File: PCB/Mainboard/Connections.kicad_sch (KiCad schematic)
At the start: 37 parts, among them J10 I2C, J11 Servo 0, J12 Servo 1, J13 PW_IO_bak, J14 PW_IO_bak, J15 Servo 4, J16 Servo 5, J17 Servo 2, J18 Servo 3, J19 Servo 6, J2 BME680, J20 Servo 7, J3 GPIO, J4 PW_5V, J5 PW_3V3, J6 Micro_SD_Card_Det_Hirose_DM3AT, J7 Stepper_1, J8 Stepper_2, J9 SPI

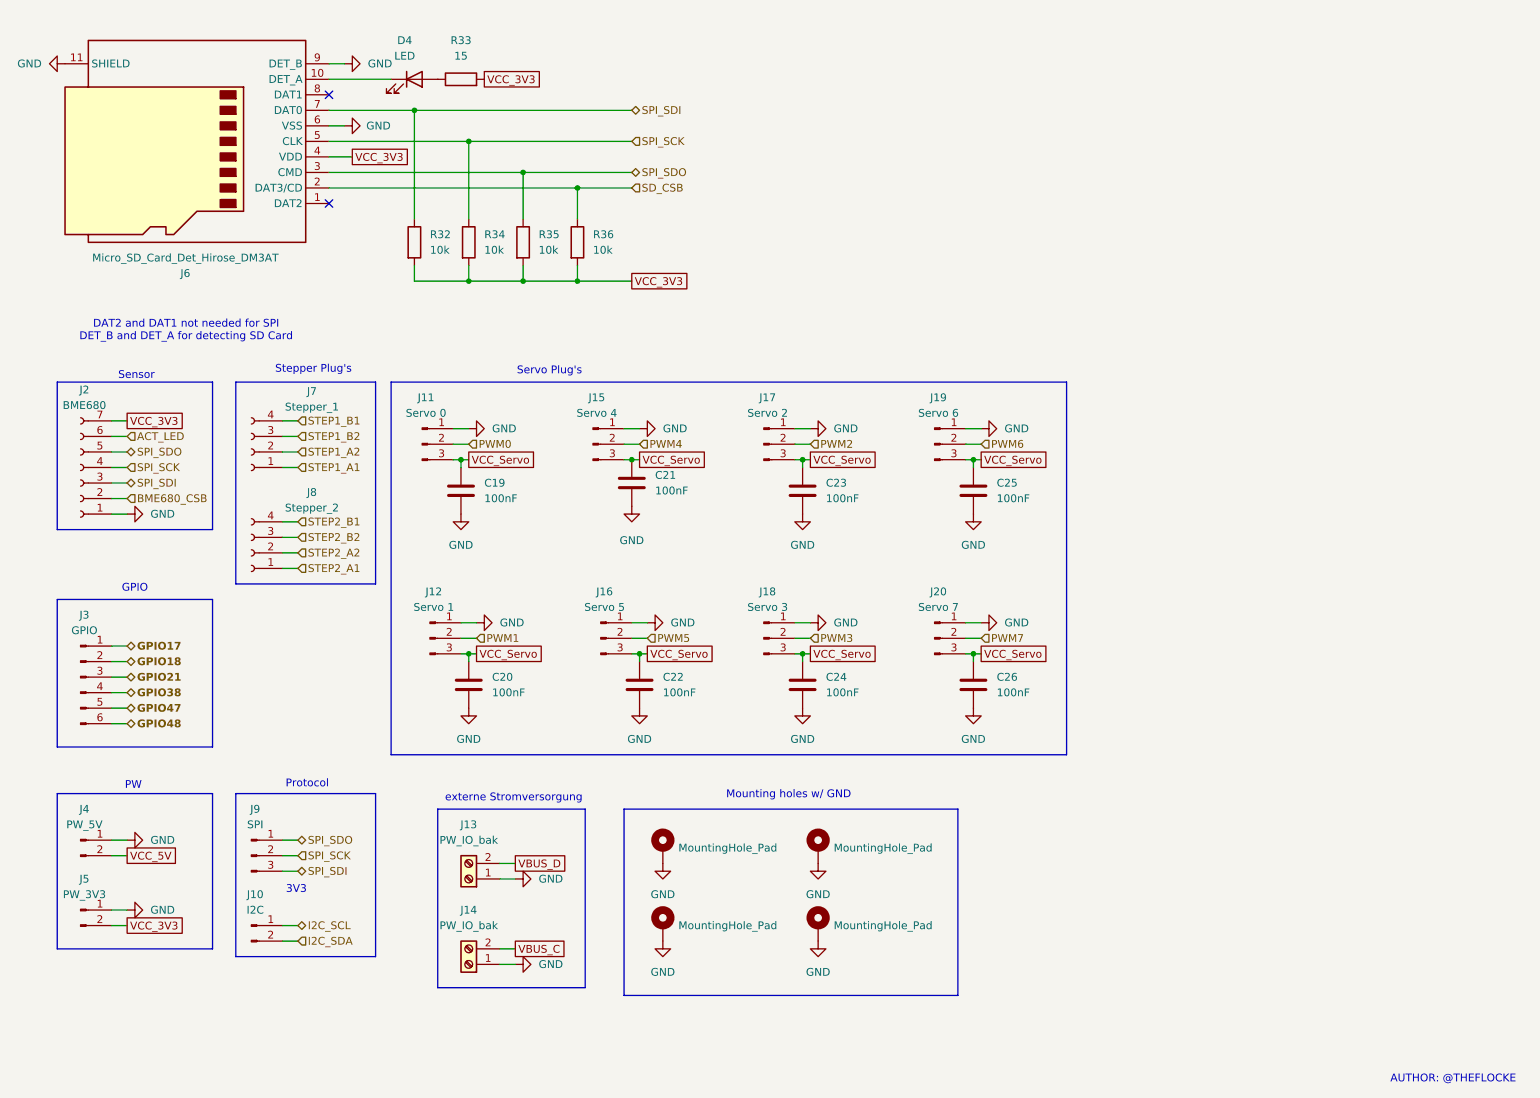
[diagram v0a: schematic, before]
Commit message: Fixed Grammar
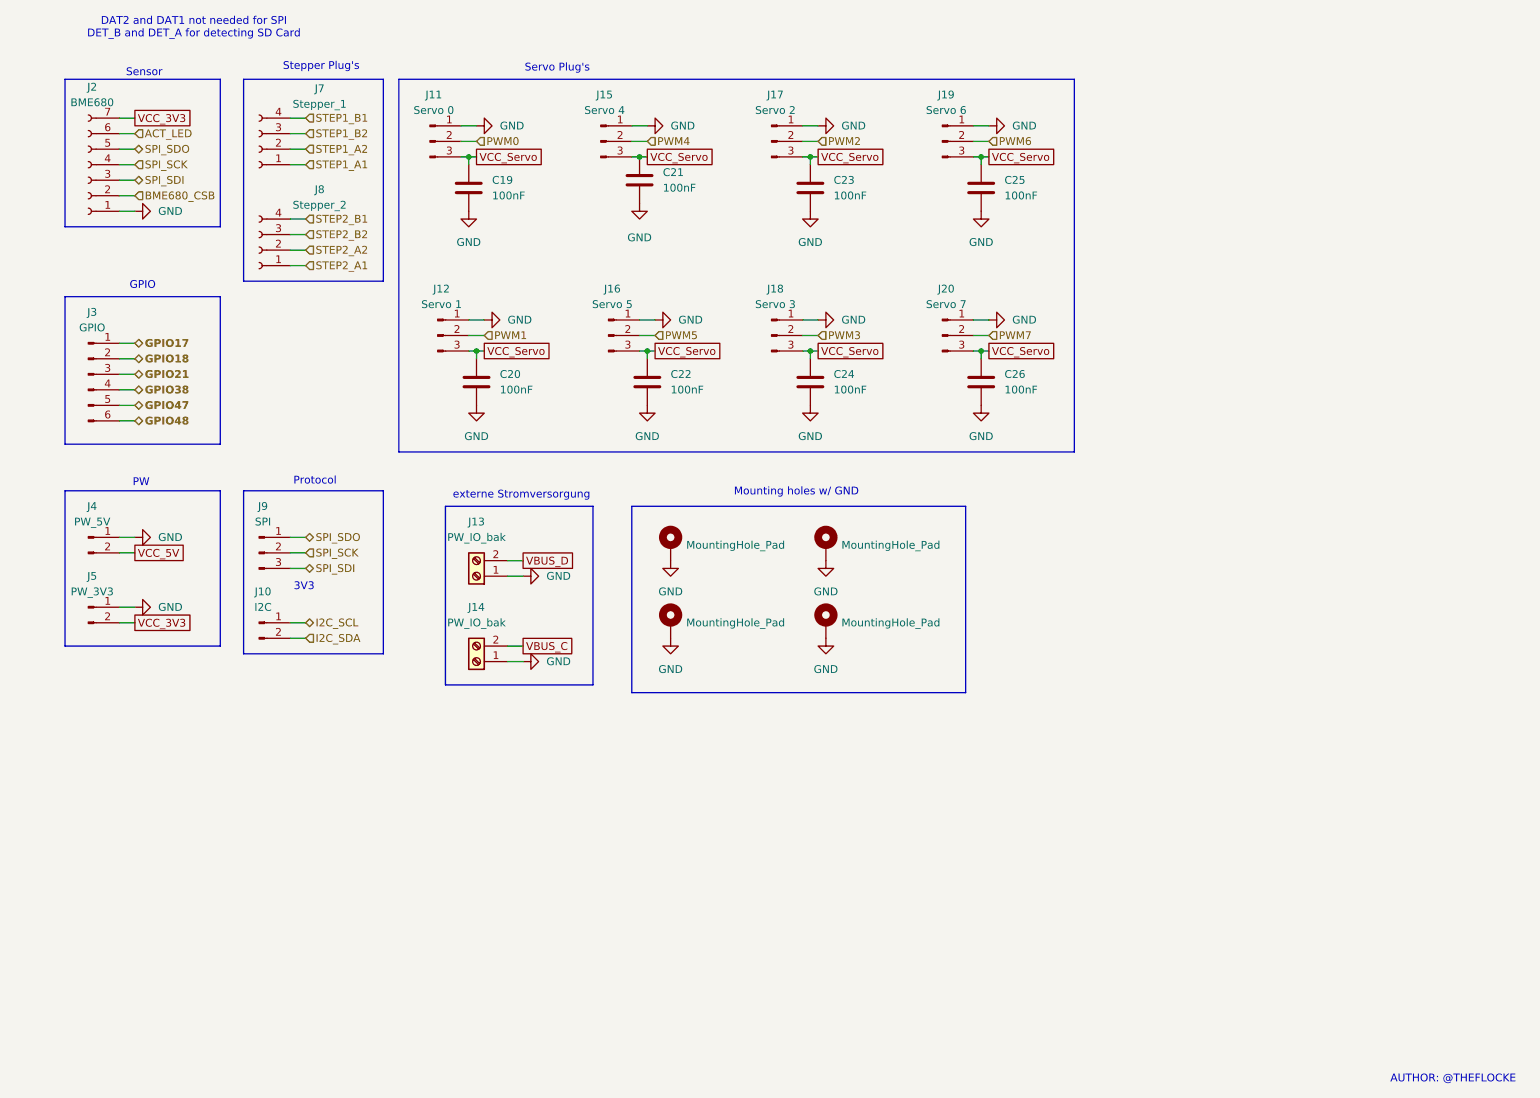
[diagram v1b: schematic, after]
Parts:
- removed D4: LED, Diode_SMD:D_0805_2012Metric_Pad1.15x1.40mm_HandSolder, symbol Device:LED
- removed J6: Micro_SD_Card_Det_Hirose_DM3AT, Connector_Card:microSD_HC_Hirose_DM3D-SF, symbol Connector:Micro_SD_Card_Det_Hirose_DM3AT
- removed R32, R34, R35, R36: 10k, Resistor_SMD:R_0805_2012Metric_Pad1.20x1.40mm_HandSolder, symbol Device:R
- removed R33: 15, Resistor_SMD:R_0805_2012Metric_Pad1.20x1.40mm_HandSolder, symbol Device:R
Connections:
- no-connect marks 2 -> 0
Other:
- moved on the sheet: C19, C20, C21, C22, C23, C24, C25, C26, J10, J11, J12, J13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

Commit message: upload images and deleted pcb new
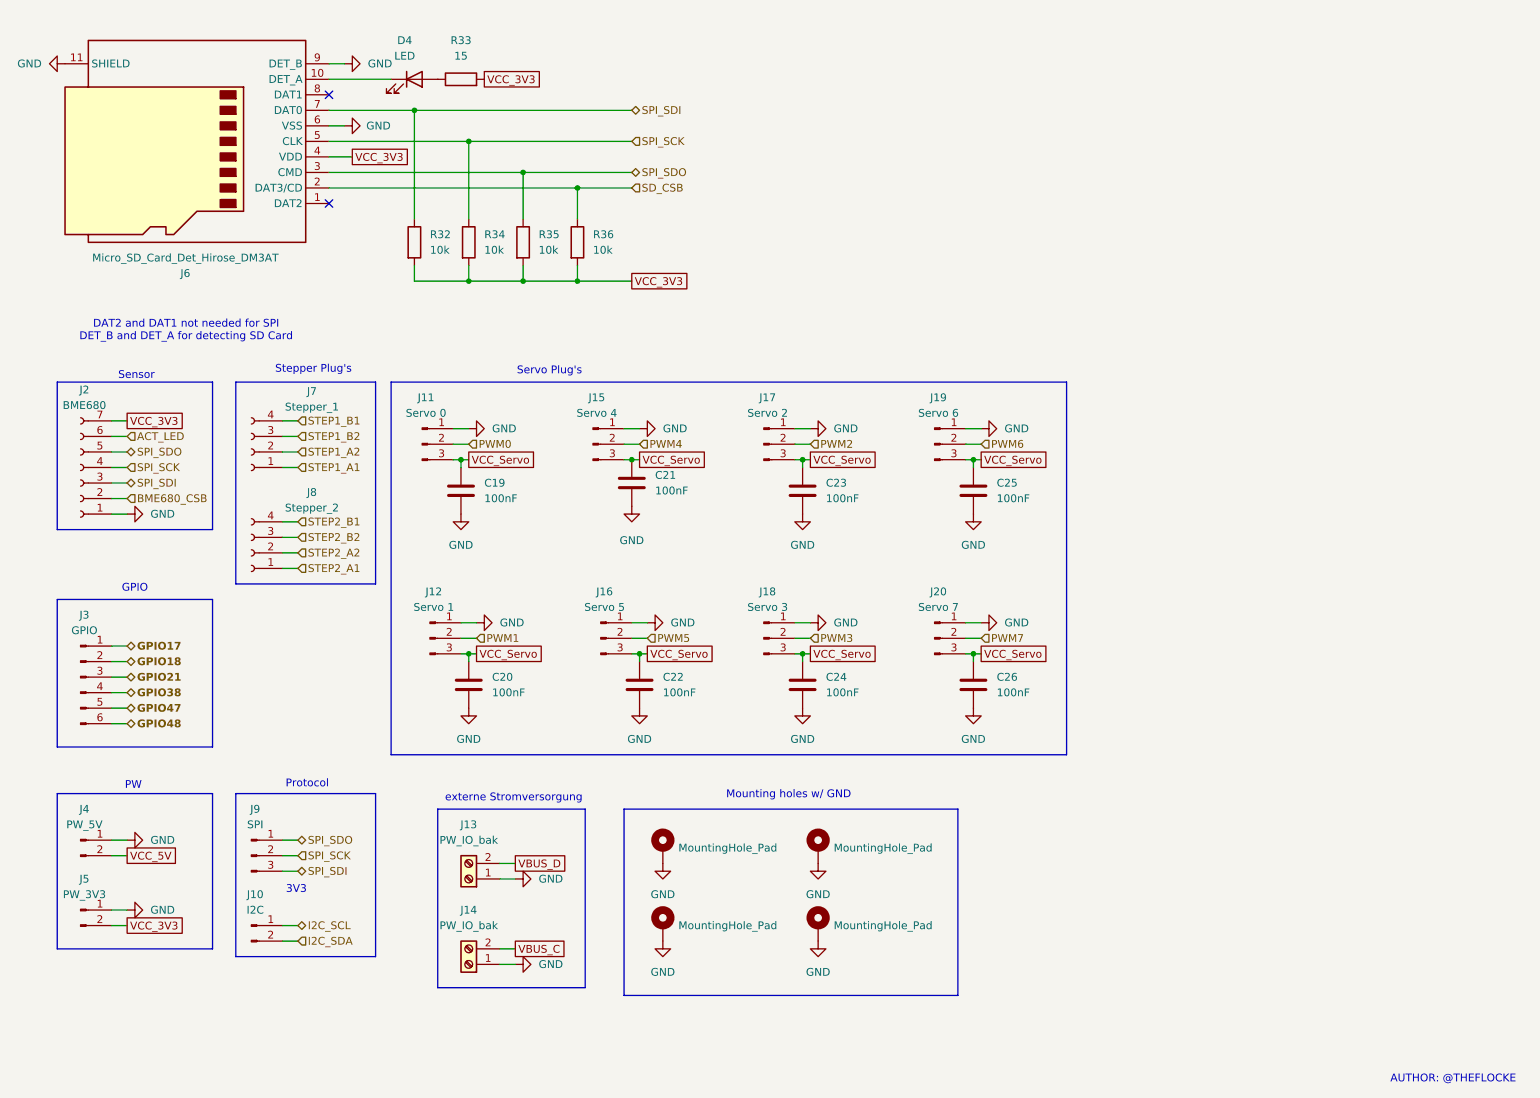
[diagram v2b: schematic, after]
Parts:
- added D4: LED, Diode_SMD:D_0805_2012Metric_Pad1.15x1.40mm_HandSolder, symbol Device:LED
- added J6: Micro_SD_Card_Det_Hirose_DM3AT, Connector_Card:microSD_HC_Hirose_DM3D-SF, symbol Connector:Micro_SD_Card_Det_Hirose_DM3AT
- added R32, R34, R35, R36: 10k, Resistor_SMD:R_0805_2012Metric_Pad1.20x1.40mm_HandSolder, symbol Device:R
- added R33: 15, Resistor_SMD:R_0805_2012Metric_Pad1.20x1.40mm_HandSolder, symbol Device:R
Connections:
- net GND: now also J6.11 (SHIELD), J6.6 (VSS), J6.9 (DET_B)
- net SPI_SCK: now also J6.5 (CLK), R34.1
- net SPI_SDI: now also J6.7 (DAT0), R32.1
- net SPI_SDO: now also J6.3 (CMD), R35.1
- net VCC_3V3: now also J6.4 (VDD), R32.2, R33.2, R34.2, R35.2, R36.2
- new net: D4.1 (K), J6.10 (DET_A)
- new net: D4.2 (A), R33.1
- new net SD_CSB: J6.2 (DAT3/CD), R36.1
- no-connect marks 0 -> 2
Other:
- moved on the sheet: C19, C20, C21, C22, C23, C24, C25, C26, J10, J11, J12, J13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
